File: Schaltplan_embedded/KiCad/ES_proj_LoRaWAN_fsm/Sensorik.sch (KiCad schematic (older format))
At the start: 27 parts, among them IC1 TPS22943DCKR, IC2 BGA824N6E6327XTSA1, IC3 TESEO-LIV3F, J3 53048-0810, J4 CONSMA002-L-G, J5 CONSMA002-L-G, U2 RFM92W_93W

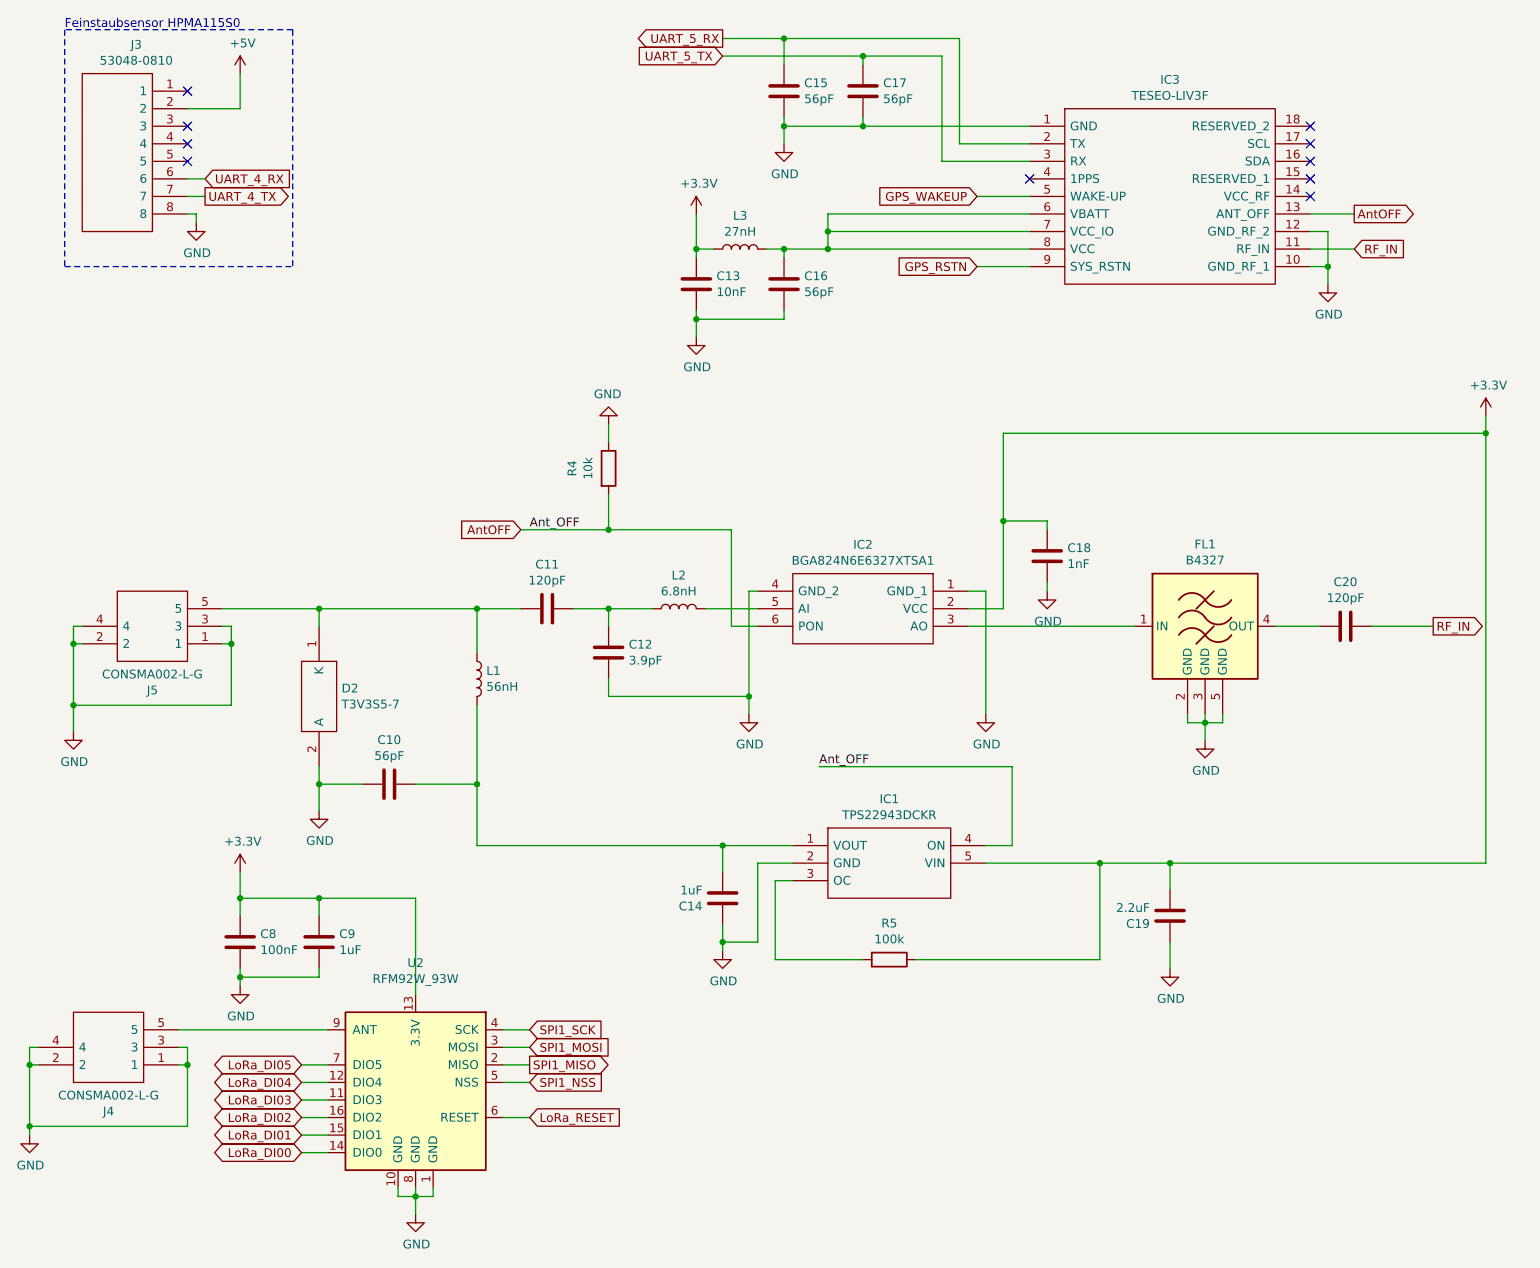
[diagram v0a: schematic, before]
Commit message: git :)
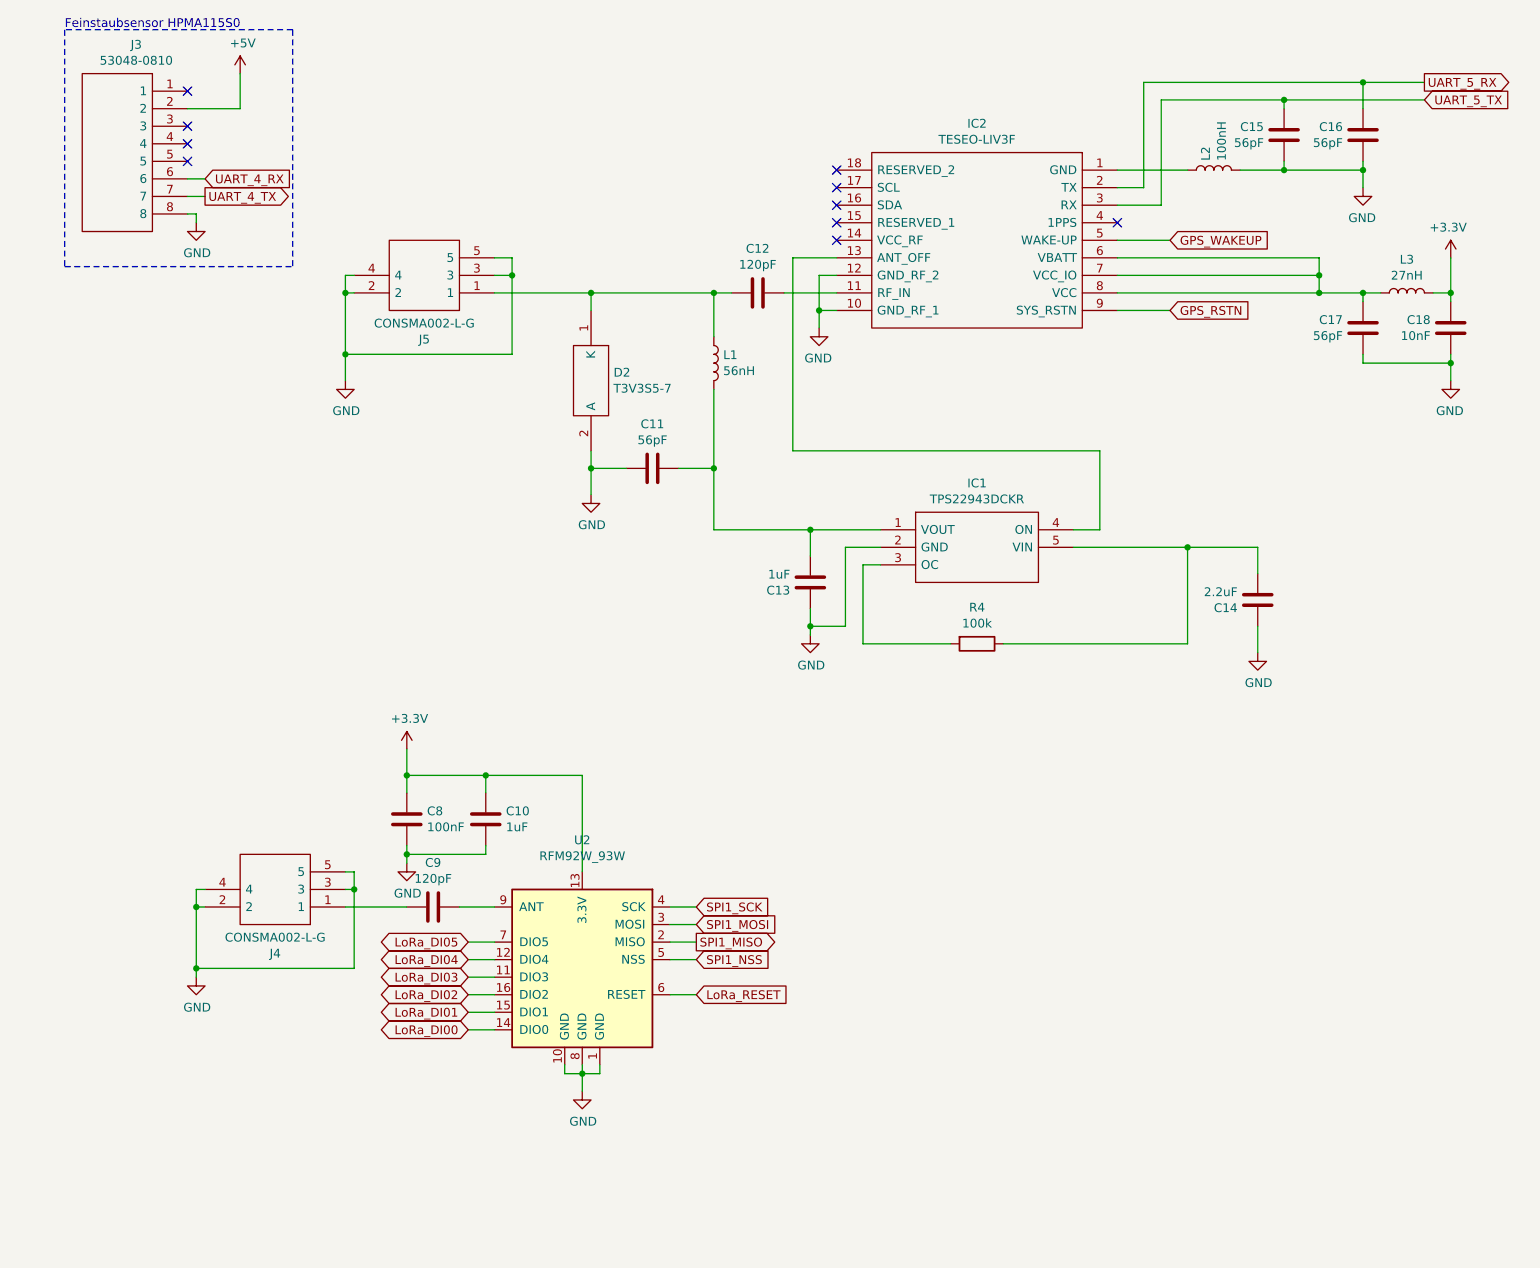
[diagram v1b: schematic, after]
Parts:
- removed C11: 120pF, Capacitors_SMD:C_0805_HandSoldering, symbol Device:C
- removed C18: 1nF, Capacitors_SMD:C_0805, symbol Device:C
- removed C20: 120pF, Capacitors_SMD:C_0805, symbol Device:C
- removed FL1: B4327, SamacSys_Parts:B39162B4353P810, symbol Schaltplan_embedded-rescue:B4327-RF_Filter_neu-Schaltplan_embedded-rescue
- removed IC2: BGA824N6E6327XTSA1, SamacSys_Parts:BGA725L6E6327, symbol SamacSys_Parts:BGA824N6E6327XTSA1
- removed R4: 10k, Resistors_SMD:R_0805_HandSoldering, symbol Device:R
- added C9: 120pF, Capacitor_SMD:C_0805_2012Metric_Pad1.15x1.40mm_HandSolder, symbol Device:C
- C12: value 3.9pF -> 120pF; footprint Capacitors_SMD:C_0805 -> Capacitor_SMD:C_0805_2012Metric_Pad1.15x1.40mm_HandSolder
- C13: renamed from C14; footprint Capacitors_SMD:C_0805 -> Capacitor_SMD:C_0805_2012Metric_Pad1.15x1.40mm_HandSolder
- C14: renamed from C19; footprint Capacitors_SMD:C_0805 -> Capacitor_SMD:C_0805_2012Metric_Pad1.15x1.40mm_HandSolder
- C15: renamed from C17; footprint Capacitors_SMD:C_0805 -> Capacitor_SMD:C_0805_2012Metric_Pad1.15x1.40mm_HandSolder
- C16: renamed from C15; footprint Capacitors_SMD:C_0805 -> Capacitor_SMD:C_0805_2012Metric_Pad1.15x1.40mm_HandSolder
- C17: renamed from C16; footprint Capacitors_SMD:C_0805 -> Capacitor_SMD:C_0805_2012Metric_Pad1.15x1.40mm_HandSolder
- C18: renamed from C13; footprint Capacitors_SMD:C_0805 -> Capacitor_SMD:C_0805_2012Metric_Pad1.15x1.40mm_HandSolder
- L1, L3: footprint Resistors_SMD:R_0805_HandSoldering -> Inductor_SMD:L_0805_2012Metric_Pad1.15x1.40mm_HandSolder
- L2: value 6.8nH -> 100nH; footprint Resistors_SMD:R_0805_HandSoldering -> Inductor_SMD:L_0805_2012Metric_Pad1.15x1.40mm_HandSolder
- renumbered C9 to C10, C10 to C11, IC3 to IC2, R5 to R4
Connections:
- net +3V3: no longer C14.1, IC1.5 (VIN), R4.1
- net GND: now also J4.5, J5.5, L2.2; no longer C12.1, IC2.1 (GND), J4.1, J5.1
- net at D2.1 (K), L1.1: now also C12.2, J5.1; no longer J5.5
- net at L2.1: now also IC2.1 (GND); no longer C12.2
- net at U2.9 (ANT): now also C9.1; no longer J4.5
- net AntOFF: no longer names the net of IC1.4 (ON), IC2.13 (ANT_OFF)
- net RF_IN: no longer names the net of IC2.11 (RF_IN)
- net RF_IN: now also C12.1
- new net: C14.1, IC1.5 (VIN), R4.1
- new net: C9.2, J4.1
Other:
- moved on the sheet: C10, C11, C13, C14, C15, C16, C17, C18, C8, D2, IC1, IC2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
